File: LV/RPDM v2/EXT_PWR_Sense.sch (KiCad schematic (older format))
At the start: 3 parts, among them K3 J115F

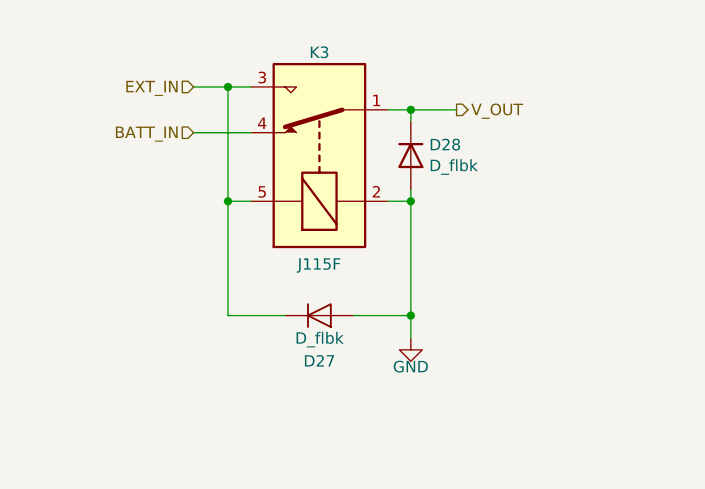
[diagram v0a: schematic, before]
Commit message: rPDM - Started on board layout
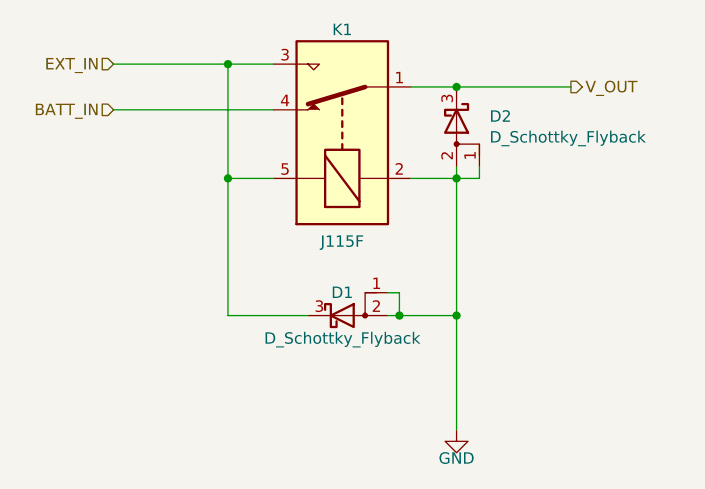
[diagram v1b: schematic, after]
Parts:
- removed D27: D_flbk, symbol Device:D
- removed D28: D_flbk, symbol Device2:D
- added D1, D2: D_Schottky_Flyback, Diode_UOWM:TO-277_FSV10150V, symbol Device2:D_Schottky_AAK
- renumbered K3 to K1
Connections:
- net EXT_IN: now also D1.3 (K)
- net GND: now also D1.1 (A), D1.2 (A), D2.1 (A), D2.2 (A)
- net V_OUT: now also D2.3 (K)
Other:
- moved on the sheet: K1
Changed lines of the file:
@@
 $Descr A4 11693 8268
 encoding utf-8
-Sheet 29 32
+Sheet 2 32
 Title ""
 Date ""
@@
 L Relay:G5LE-1 K?
 U 1 1 60E948E2
-P 5400 3300
+P 5500 3200
 AR Path="/5E554D5D/60E948E2" Ref="K?"  Part="1"
 AR Path="/5E554D5D/5E5E9CA9/60E948E2" Ref="K?"  Part="1"
@@
 AR Path="/60E5EBEF/60E948E2" Ref="K?"  Part="1"
 AR Path="/60E948E2" Ref="K?"  Part="1"
-AR Path="/60E91844/60E948E2" Ref="K3"  Part="1"
-F 0 "K3" V 5850 3300 50  0000 C CNN
-F 1 "J115F" V 4924 3300 50  0000 C CNN
-F 2 "" H 5850 3250 50  0001 L CNN
-F 3 "" H 5400 3300 50  0001 C CNN
-	1    5400 3300
+AR Path="/60E91844/60E948E2" Ref="K1"  Part="1"
+F 0 "K1" V 5950 3200 50  0000 C CNN
+F 1 "J115F" V 5024 3200 50  0000 C CNN
+F 2 "" H 5950 3150 50  0001 L CNN
+F 3 "" H 5500 3200 50  0001 C CNN
+	1    5500 3200
 	0    -1   -1   0
 $EndComp
-$Comp
-L Device:D D?
-U 1 1 60E948E8
-P 5400 4000
-AR Path="/5E554D5D/60E948E8" Ref="D?"  Part="1"
-AR Path="/5E554D5D/5E5E9CA9/60E948E8" Ref="D?"  Part="1"
-AR Path="/5E554D5D/5E5A0290/60E948E8" Ref="D?"  Part="1"
-AR Path="/5E554D5D/5E5A035E/60E948E8" Ref="D?"  Part="1"
-AR Path="/5E554D5D/5E5A09AA/60E948E8" Ref="D?"  Part="1"
-AR Path="/5E554D5D/5E5A0BF4/60E948E8" Ref="D?"  Part="1"
-AR Path="/5E554D5D/610FDB0E/60E948E8" Ref="D?"  Part="1"
-AR Path="/5E554D5D/60DE75D7/60E948E8" Ref="D?"  Part="1"
-AR Path="/5E554D5D/60DE7B67/60E948E8" Ref="D?"  Part="1"
-AR Path="/5E554D5D/60DE7FBD/60E948E8" Ref="D?"  Part="1"
-AR Path="/5E554D5D/60DE88EB/60E948E8" Ref="D?"  Part="1"
-AR Path="/5E554D5D/60DED789/60E948E8" Ref="D?"  Part="1"
-AR Path="/5E554D5D/60DEDCB5/60E948E8" Ref="D?"  Part="1"
-AR Path="/60E5EBEF/60E948E8" Ref="D?"  Part="1"
-AR Path="/60E948E8" Ref="D?"  Part="1"
-AR Path="/60E91844/60E948E8" Ref="D27"  Part="1"
-F 0 "D27" H 5400 4200 50  0000 C CNN
-F 1 "D_flbk" H 5400 4100 50  0000 C CNN
-F 2 "" H 5400 4000 50  0001 C CNN
-F 3 "~" H 5400 4000 50  0001 C CNN
-	1    5400 4000
-	1    0    0    1
-$EndComp
 Wire Wire Line
-	5550 4000 5800 4000
+	6000 3400 5800 3400
 Wire Wire Line
-	5800 4000 5800 3500
+	5200 3400 5000 3400
 Wire Wire Line
-	5800 3500 5700 3500
+	5000 3400 5000 4000
+Connection ~ 5000 3400
 Wire Wire Line
-	5100 3500 5000 3500
+	4500 2900 5000 2900
 Wire Wire Line
-	5000 3500 5000 4000
+	5000 2900 5000 3400
 Wire Wire Line
-	5000 4000 5250 4000
-Connection ~ 5000 3500
-Wire Wire Line
-	4850 3000 5000 3000
-Wire Wire Line
-	5000 3000 5000 3500
-Wire Wire Line
-	5100 3000 5000 3000
-Connection ~ 5000 3000
+	5200 2900 5000 2900
+Connection ~ 5000 2900
 $Comp
 L power:GND #PWR?
 U 1 1 60E948F9
-P 5800 4100
+P 6000 4500
 AR Path="/60E948F9" Ref="#PWR?"  Part="1"
-AR Path="/60E91844/60E948F9" Ref="#PWR035"  Part="1"
-F 0 "#PWR035" H 5800 3850 50  0001 C CNN
-F 1 "GND" H 5800 3975 50  0000 C CNN
-F 2 "" H 5800 4100 50  0001 C CNN
-F 3 "" H 5800 4100 50  0001 C CNN
-	1    5800 4100
+AR Path="/60E91844/60E948F9" Ref="#PWR04"  Part="1"
+F 0 "#PWR04" H 6000 4250 50  0001 C CNN
+F 1 "GND" H 6000 4375 50  0000 C CNN
+F 2 "" H 6000 4500 50  0001 C CNN
+F 3 "" H 6000 4500 50  0001 C CNN
+	1    6000 4500
+	1    0    0    -1
+$EndComp
+Text HLabel 4500 2900 0    50   Input ~ 0
+EXT_IN
+Wire Wire Line
+	5200 3100 4500 3100
+Text HLabel 4500 3100 0    50   Input ~ 0
+BATT_IN
+Text HLabel 6500 3000 2    50   Output ~ 0
+V_OUT
+$Comp
+L Device2:D_Schottky_AAK D?
+U 1 1 619864CC
+P 6000 3150
+AR Path="/5E554D5D/60DED789/619864CC" Ref="D?"  Part="1"
+AR Path="/5E554D5D/5E5E9CA9/619864CC" Ref="D?"  Part="1"
+AR Path="/60E91844/619864CC" Ref="D2"  Part="1"
+F 0 "D2" V 5979 3294 50  0000 L CNN
+F 1 "D_Schottky_Flyback" V 6070 3294 50  0000 L CNN
+F 2 "Diode_UOWM:TO-277_FSV10150V" H 6000 3150 50  0001 C CNN
+F 3 "~" H 6000 3150 50  0001 C CNN
+	1    6000 3150
+	0    1    1    0
+$EndComp
+$Comp
+L Device2:D_Schottky_AAK D?
+U 1 1 6198713A
+P 5500 4000
+AR Path="/5E554D5D/60DED789/6198713A" Ref="D?"  Part="1"
+AR Path="/5E554D5D/5E5E9CA9/6198713A" Ref="D?"  Part="1"
+AR Path="/60E91844/6198713A" Ref="D1"  Part="1"
+F 0 "D1" H 5500 4100 50  0000 C CNN
+F 1 "D_Schottky_Flyback" H 5500 3900 50  0000 C CNN
+F 2 "Diode_UOWM:TO-277_FSV10150V" H 5500 4000 50  0001 C CNN
+F 3 "~" H 5500 4000 50  0001 C CNN
+	1    5500 4000
 	1    0    0    -1
 $EndComp
 Wire Wire Line
-	5800 4100 5800 4000
-Connection ~ 5800 4000
+	6000 3400 6000 4000
+Connection ~ 6000 3400
 Wire Wire Line
-	5700 3100 5800 3100
-Text HLabel 4850 3000 0    50   Input ~ 0
-EXT_IN
+	5000 4000 5350 4000
 Wire Wire Line
-	5100 3200 4850 3200
-Text HLabel 4850 3200 0    50   Input ~ 0
-BATT_IN
-Text HLabel 6000 3100 2    50   Output ~ 0
-V_OUT
-$Comp
-L Device2:D D28
-U 1 1 61712BAF
-P 5800 3300
-F 0 "D28" V 5754 3380 50  0000 L CNN
-F 1 "D_flbk" V 5845 3380 50  0000 L CNN
-F 2 "" H 5800 3300 50  0001 C CNN
-F 3 "~" H 5800 3300 50  0001 C CNN
-	1    5800 3300
-	0    1    1    0
-$EndComp
+	5700 4000 5750 4000
+Connection ~ 6000 4000
 Wire Wire Line
-	5800 3150 5800 3100
-Connection ~ 5800 3100
+	6000 4000 6000 4500
 Wire Wire Line
-	5800 3100 6000 3100
+	5700 3900 5750 3900
 Wire Wire Line
-	5800 3450 5800 3500
-Connection ~ 5800 3500
+	5750 3900 5750 4000
+Connection ~ 5750 4000
+Wire Wire Line
+	5750 4000 6000 4000
+Wire Wire Line
+	5800 3000 6000 3000
+Connection ~ 6000 3000
+Wire Wire Line
+	6000 3000 6500 3000
+Wire Wire Line
+	6000 3350 6000 3400
+Wire Wire Line
+	6100 3350 6100 3400
+Wire Wire Line
+	6100 3400 6000 3400
 $EndSCHEMATC
